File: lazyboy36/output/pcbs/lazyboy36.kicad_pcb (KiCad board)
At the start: 2 copper layers, 211.8 x 146.1 mm, 83 parts

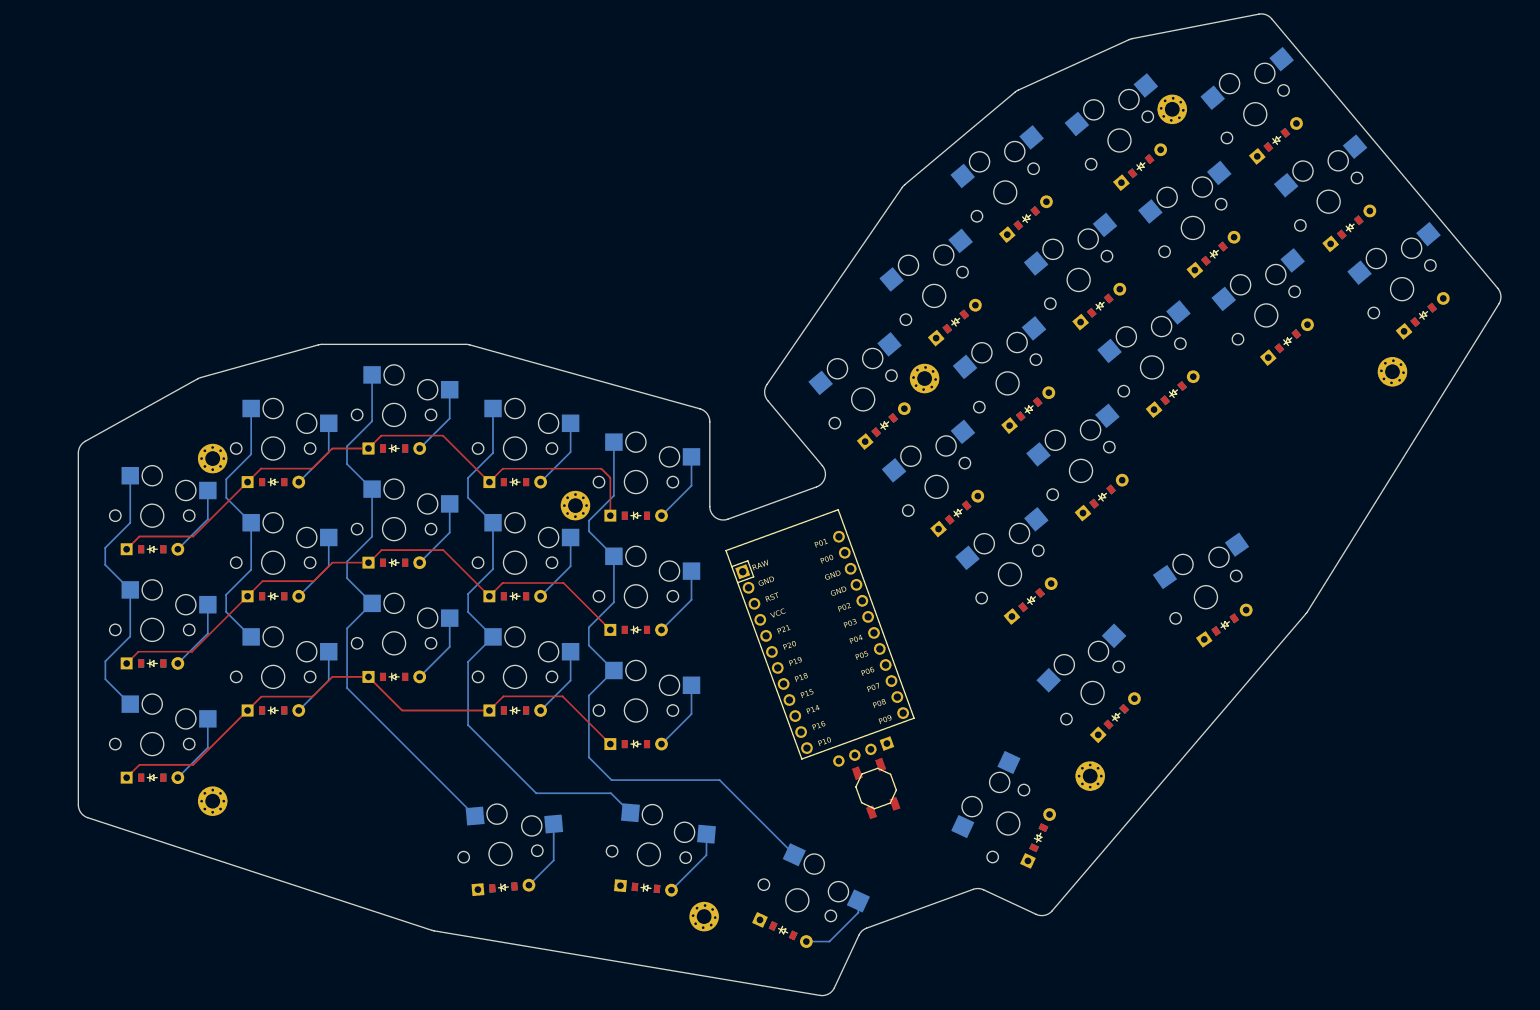
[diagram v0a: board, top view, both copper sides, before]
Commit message: 완성
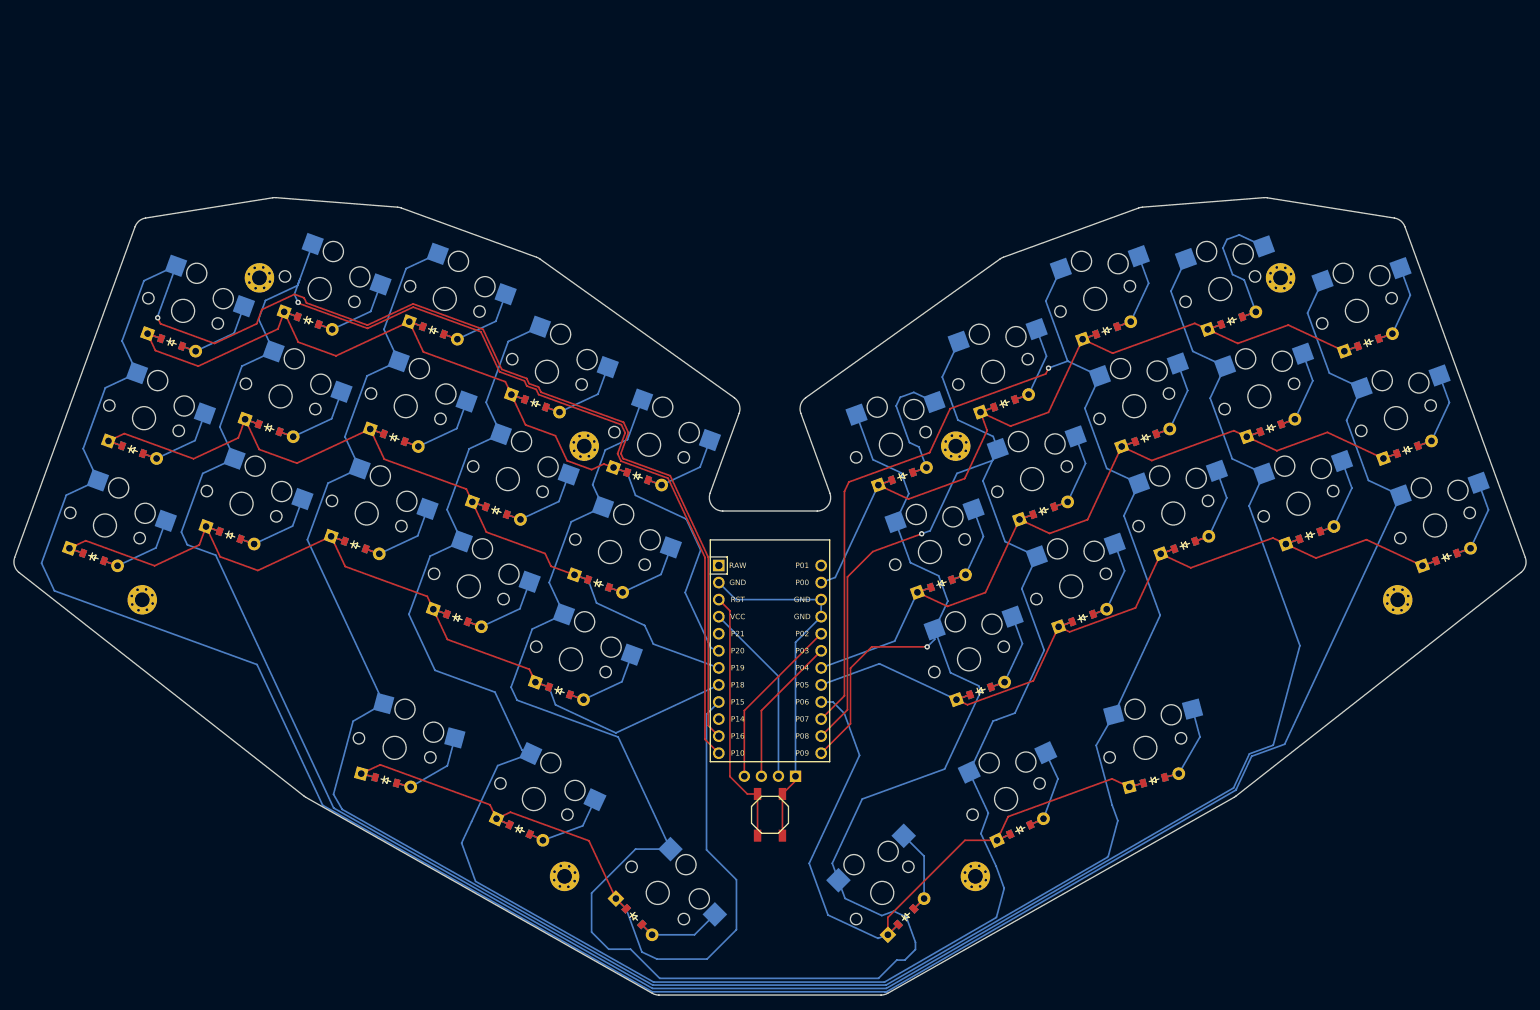
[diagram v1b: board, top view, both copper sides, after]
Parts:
- moved D19 36.2 mm to (256.5, 134.5), turned to 20 degrees
- moved S19 35.5 mm to (254.7, 129.8), turned to 20 degrees
- moved D20 34.2 mm to (250.6, 118.6), turned to 20 degrees
- moved D1 34.0 mm to (55.0, 134.5), turned to -20 degrees
- moved _6 34.0 mm to (249.2, 140.9), turned to 20 degrees
- moved S20 33.7 mm to (248.9, 113.9), turned to 20 degrees
- moved S1 33.3 mm to (56.7, 129.8), turned to -20 degrees
- moved D21 33.1 mm to (244.8, 102.6), turned to 20 degrees
- moved S21 33.0 mm to (243.1, 97.9), turned to 20 degrees
- moved D2 32.0 mm to (60.9, 118.6), turned to -20 degrees
- moved _2 31.8 mm to (62.3, 140.9), turned to -20 degrees
- moved S2 31.5 mm to (62.6, 113.9), turned to -20 degrees
- moved D3 30.9 mm to (66.7, 102.6), turned to -20 degrees
- moved S3 30.8 mm to (68.4, 97.9), turned to -20 degrees
- moved _5 29.8 mm to (231.7, 93.0), turned to 20 degrees
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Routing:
- net P16: track 40.2 -> 502.8 mm, vias 0 -> 1
- net P10: track 40.2 -> 460.3 mm, vias 0 -> 1
- net P7: track 81.3 -> 402.4 mm, vias 0 -> 1
- net P8: track 84.4 -> 349.9 mm, vias 0 -> 1
- net P9: track 91.2 -> 302.4 mm, vias 0 -> 1
- net P4: track 0.00 -> 129.4 mm
- net P0: track 0.00 -> 128.9 mm
- net P5: track 0.00 -> 128.0 mm
- net P15: track 0.00 -> 119.4 mm
- net P6: track 0.00 -> 106.2 mm
- net P20: track 88.9 -> 145.4 mm
- net P18: track 84.1 -> 137.9 mm
- net GND: track 0.00 -> 53.8 mm
- net P19: track 85.7 -> 133.3 mm
- net RST: track 0.00 -> 38.4 mm
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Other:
- board size 211.8 x 146.1 mm -> 225.1 x 118.7 mm
